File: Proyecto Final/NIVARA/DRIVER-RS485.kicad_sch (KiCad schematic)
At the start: 1 part, among them U3 MAX3485

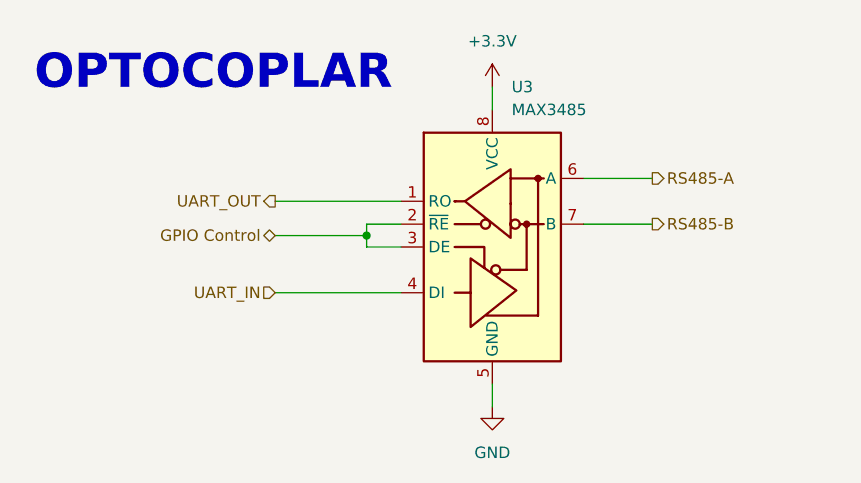
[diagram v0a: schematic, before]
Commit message: Actualización.
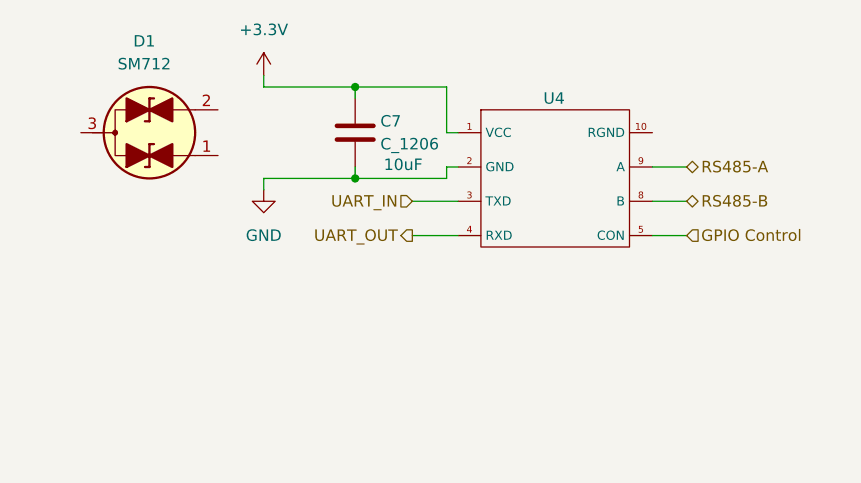
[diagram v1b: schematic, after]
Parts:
- removed U3: MAX3485, Package_SO:SOIC-8_3.9x4.9mm_P1.27mm, symbol Interface_UART:MAX3485
- added C7: C_1206, PCM_Capacitor_SMD_AKL:C_1206_3216Metric, symbol PCM_Capacitor_AKL:C_1206
- added D1: SM712, PCM_Package_TO_SOT_SMD_AKL:SOT-23, symbol PCM_Diode_TVS_AKL:SM712
- added U4: ~, Package_DIP:C2992406, symbol Interface_UART:C2992406
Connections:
- net +3.3V: now also C7.1, U4.1 (VCC)
- net GND: now also C7.2, U4.2 (GND)
- net GPIO Control: now also U4.5 (CON)
- net RS485-A: now also U4.9 (A)
- net RS485-B: now also U4.8 (B)
- net UART_IN: now also U4.3 (TXD)
- net UART_OUT: now also U4.4 (RXD)
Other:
- note removed: "OPTOCOPLAR"
